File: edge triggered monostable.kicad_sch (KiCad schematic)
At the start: 14 parts, among them J1 Screw_Terminal_01x02, J2 Screw_Terminal_01x06, J3 Screw_Terminal_01x02, K1 G5V-2, U1 NE555D

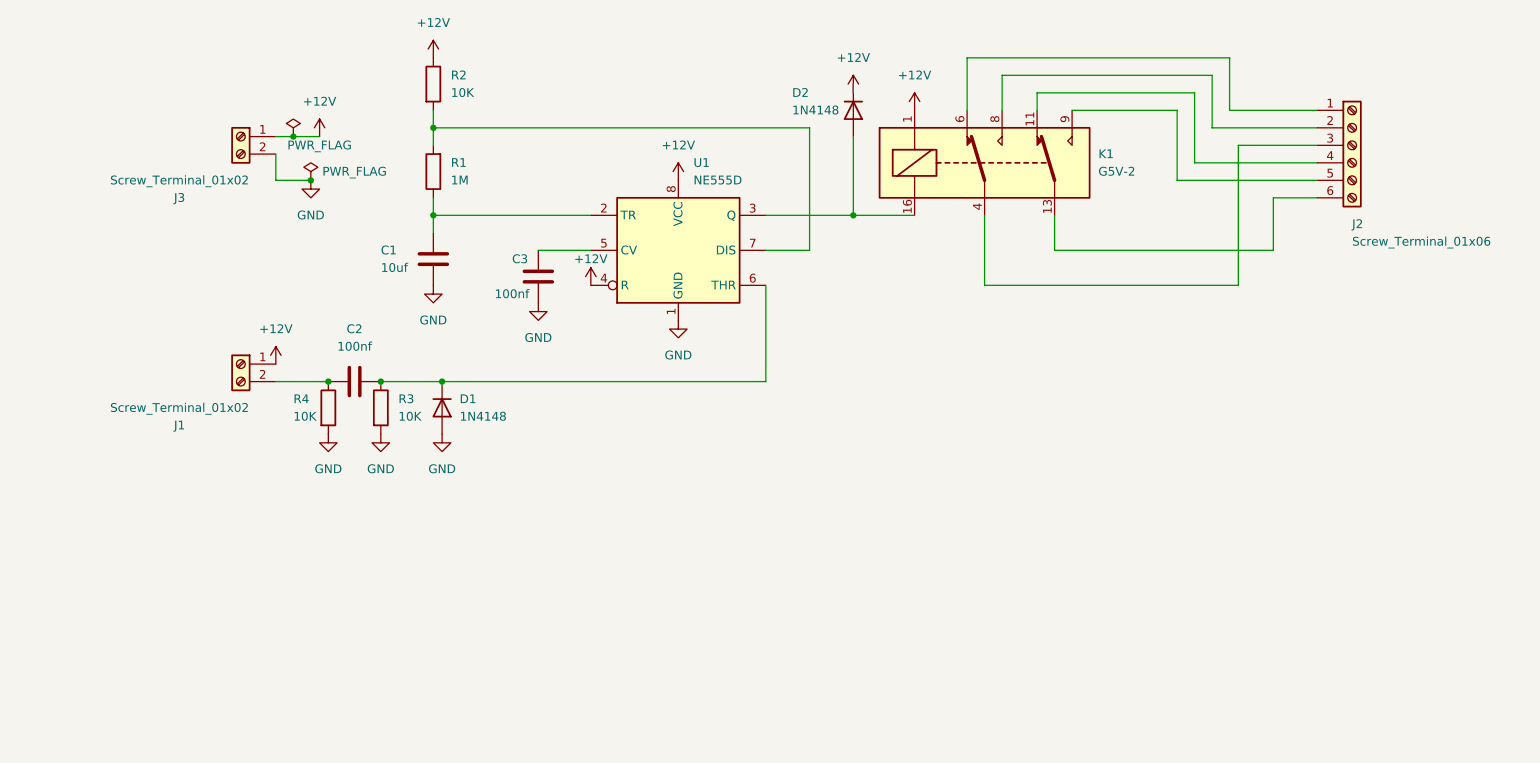
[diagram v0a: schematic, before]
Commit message: Added LED, BOM, and position files...
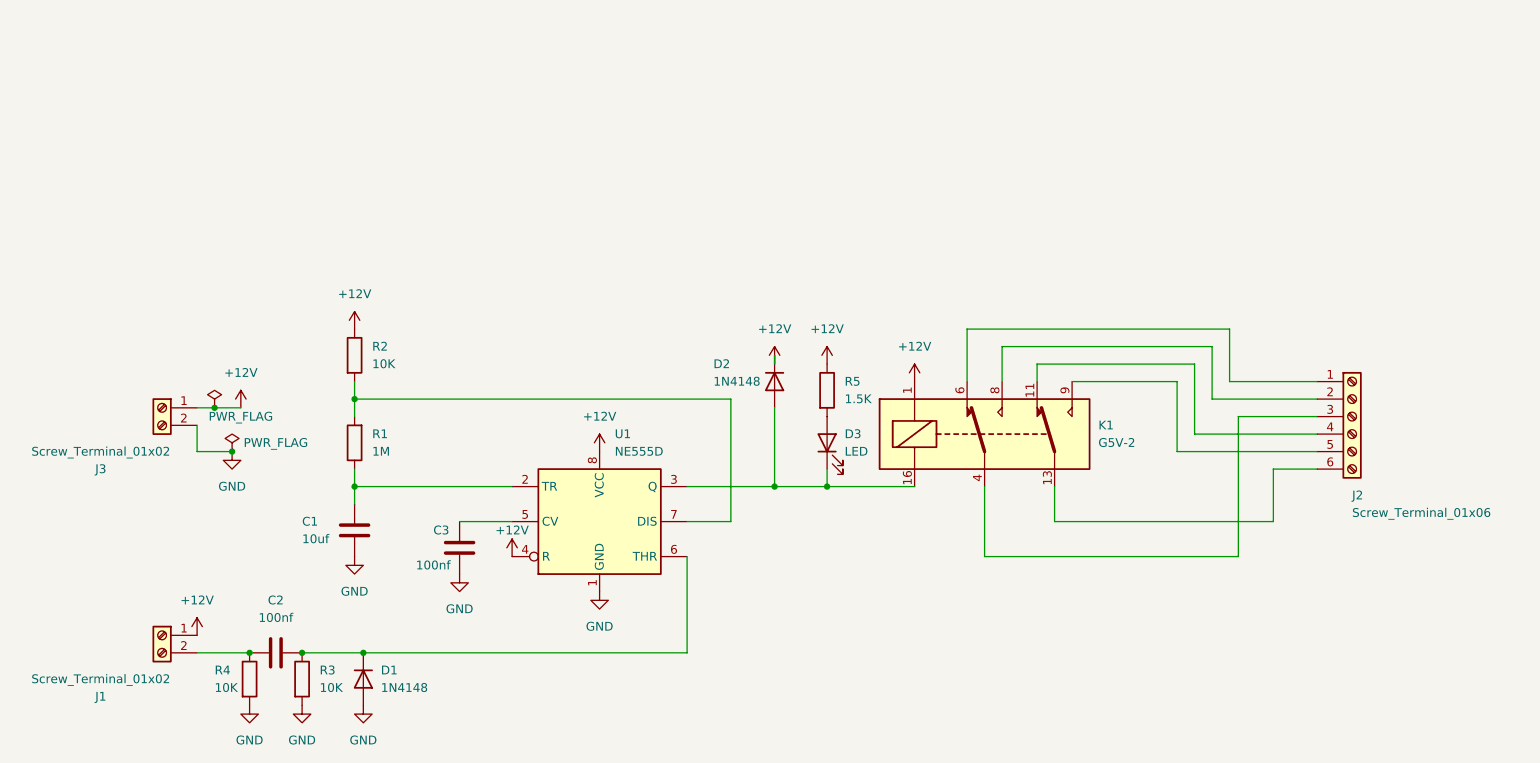
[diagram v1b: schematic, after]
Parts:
- added D3: LED, LED_SMD:LED_0805_2012Metric, symbol Device:LED
- added R5: 1.5K, Resistor_SMD:R_0805_2012Metric, symbol Device:R
- C1: LCSC (none) -> C440198
- C2, C3: LCSC (none) -> C49678
- D1, D2: LCSC (none) -> C81598
- J1, J3: LCSC (none) -> C557685
- J2: LCSC (none) -> C915915
- K1: LCSC (none) -> C28089
- R1: LCSC (none) -> C17514
- R2, R3, R4: LCSC (none) -> C17414
- U1: LCSC (none) -> C7593
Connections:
- net +12V: now also R5.1
- net at D2.2 (A), K1.16, U1.3 (Q): now also D3.1 (K)
- new net: D3.2 (A), R5.2
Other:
- moved on the sheet: C1, C2, C3, D1, D2, J1, J2, J3, K1, R1, R2, R3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
